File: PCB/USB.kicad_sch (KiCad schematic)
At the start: 7 parts, among them U20 xc7z020clg484

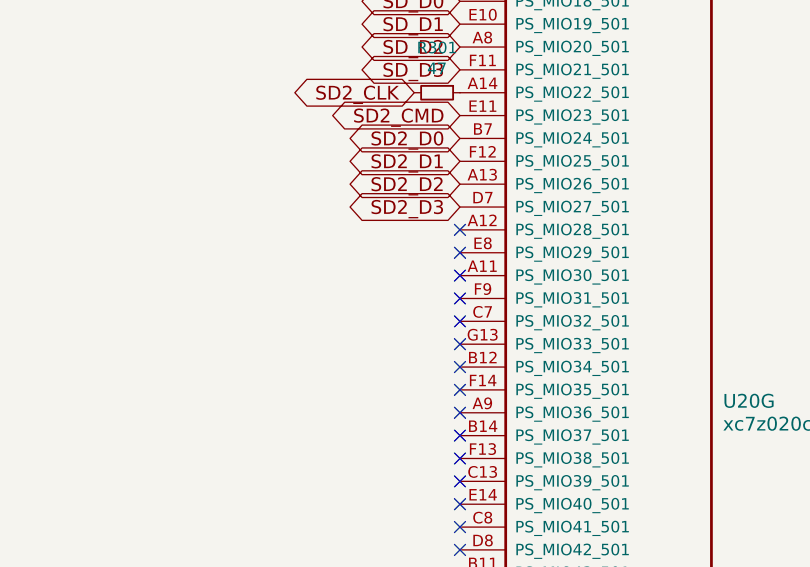
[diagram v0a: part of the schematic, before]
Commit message: some changes
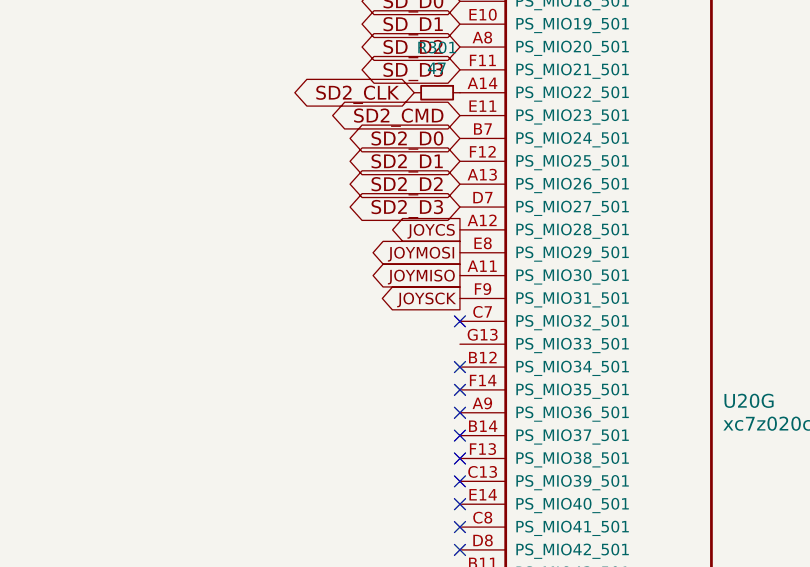
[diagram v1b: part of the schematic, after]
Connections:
- net JOYMISO: now reaches U20.A11 (PS_MIO30_501)
- net JOYCS: now reaches U20.A12 (PS_MIO28_501)
- net JOYMOSI: now reaches U20.E8 (PS_MIO29_501)
- net JOYSCK: now reaches U20.F9 (PS_MIO31_501)
- no-connect marks 27 -> 22
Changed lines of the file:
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@@
 	)
 	(no_connect
-		(at 125.095 92.71)
+		(at 125.095 128.27)
+	)
+	(no_connect
+		(at 125.095 140.97)
+	)
+	(no_connect
+		(at 125.095 133.35)
+	)
+	(no_connect
+		(at 125.095 156.21)
+	)
+	(no_connect
+		(at 125.095 125.73)
+	)
+	(no_connect
+		(at 125.095 148.59)
+	)
+	(no_connect
+		(at 125.095 123.19)
+	)
+	(no_connect
+		(at 125.095 130.81)
+	)
+	(no_connect
+		(at 125.095 115.57)
+	)
+	(no_connect
+		(at 125.095 146.05)
+	)
+	(no_connect
+		(at 125.095 120.65)
+	)
+	(no_connect
+		(at 125.095 135.89)
+	)
+	(no_connect
+		(at 125.095 143.51)
 	)
 	(no_connect
@@
 	)
 	(no_connect
-		(at 125.095 128.27)
-	)
-	(no_connect
-		(at 125.095 140.97)
-	)
-	(no_connect
-		(at 125.095 133.35)
-	)
-	(no_connect
-		(at 125.095 156.21)
-	)
-	(no_connect
-		(at 125.095 125.73)
-	)
-	(no_connect
-		(at 125.095 148.59)
-	)
-	(no_connect
-		(at 125.095 123.19)
-	)
-	(no_connect
-		(at 125.095 130.81)
-	)
-	(no_connect
-		(at 125.095 115.57)
-	)
-	(no_connect
-		(at 125.095 146.05)
-	)
-	(no_connect
-		(at 125.095 120.65)
-	)
-	(no_connect
-		(at 125.095 97.79)
-	)
-	(no_connect
-		(at 125.095 135.89)
-	)
-	(no_connect
-		(at 125.095 100.33)
-	)
-	(no_connect
-		(at 125.095 143.51)
-	)
-	(no_connect
 		(at 125.095 153.67)
 	)
 	(no_connect
 		(at 125.095 138.43)
-	)
-	(no_connect
-		(at 125.095 105.41)
-	)
-	(no_connect
-		(at 125.095 95.25)
 	)
 	(no_connect
@@
 		)
 	)
+	(global_label "JOYCS"
+		(shape output)
+		(at 125.095 92.71 180)
+		(fields_autoplaced yes)
+		(effects
+			(font
+				(size 1.27 1.27)
+			)
+			(justify right)
+		)
+		(property "Intersheetrefs" "${INTERSHEET_REFS}"
+			(at 116.8978 92.71 0)
+			(effects
+				(font
+					(size 1.27 1.27)
+				)
+				(justify right)
+				(hide yes)
+			)
+		)
+	)
 	(global_label "SD2_D3"
 		(shape bidirectional)
@@
 		)
 	)
+	(global_label "JOYSCK"
+		(shape output)
+		(at 125.095 100.33 180)
+		(fields_autoplaced yes)
+		(effects
+			(font
+				(size 1.27 1.27)
+			)
+			(justify right)
+		)
+		(property "Intersheetrefs" "${INTERSHEET_REFS}"
+			(at 115.6278 100.33 0)
+			(effects
+				(font
+					(size 1.27 1.27)
+				)
+				(justify right)
+				(hide yes)
+			)
+		)
+	)
 	(global_label "SD2_D2"
 		(shape bidirectional)
@@
 		)
 	)
+	(global_label "JOYMISO"
+		(shape output)
+		(at 125.095 97.79 180)
+		(fields_autoplaced yes)
+		(effects
+			(font
+				(size 1.27 1.27)
+			)
+			(justify right)
+		)
+		(property "Intersheetrefs" "${INTERSHEET_REFS}"
+			(at 114.7811 97.79 0)
+			(effects
+				(font
+					(size 1.27 1.27)
+				)
+				(justify right)
+				(hide yes)
+			)
+		)
+	)
 	(global_label "SD2_D1"
 		(shape bidirectional)
@@
 				(hide yes)
 			)
+		)
+	)
+	(global_label "JOYMOSI"
+		(shape output)
+		(at 125.095 95.25 180)
+		(fields_autoplaced yes)
+		(effects
+			(font
+				(size 1.27 1.27)
+			)
+			(justify right)
+		)
+		(property "Intersheetrefs" "${INTERSHEET_REFS}"
+			(at 114.7811 95.25 0)
+			(effects
+				(font
+					(size 1.27 1.27)
+				)
+				(justify right)
+				(hide yes)
+			)

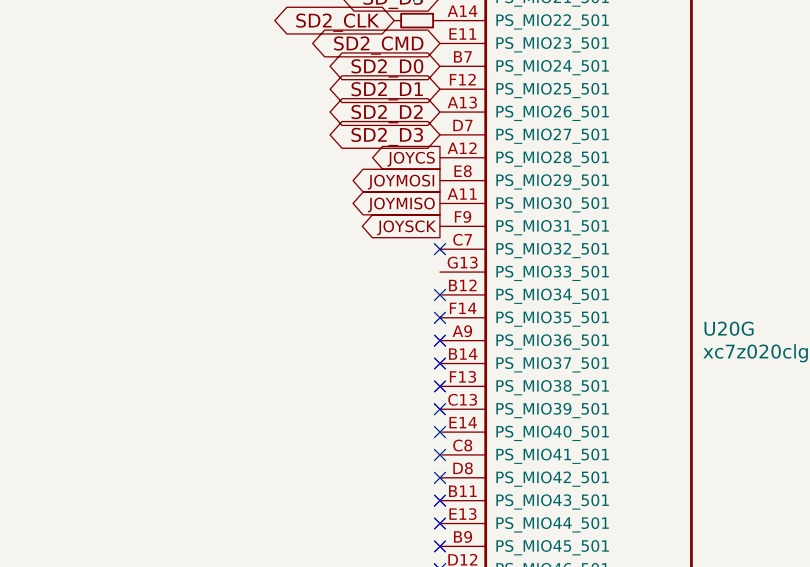
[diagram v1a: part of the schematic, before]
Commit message: [+] Layouting
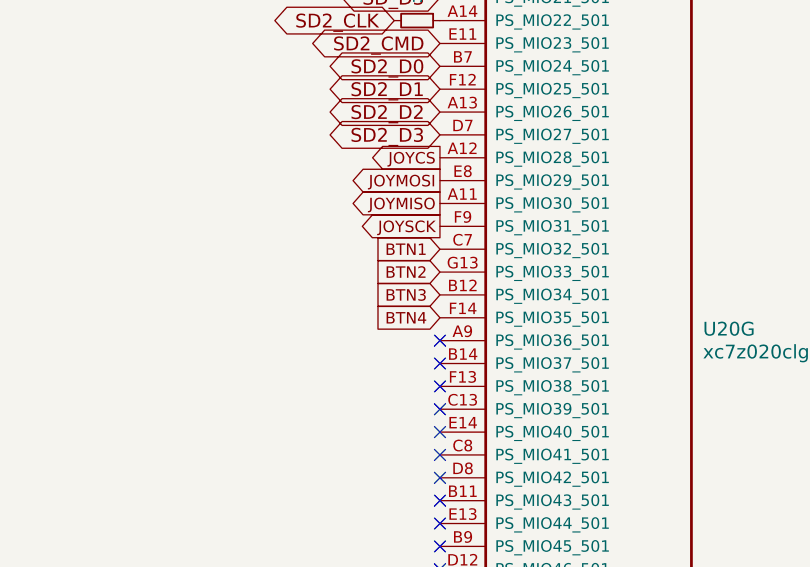
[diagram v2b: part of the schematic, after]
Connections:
- net BTN3: now reaches U20.B12 (PS_MIO34_501)
- net BTN1: now reaches U20.C7 (PS_MIO32_501)
- net BTN4: now reaches U20.F14 (PS_MIO35_501)
- net BTN2: now reaches U20.G13 (PS_MIO33_501)
- no-connect marks 22 -> 19
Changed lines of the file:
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@@
-	)
-	(no_connect
-		(at 125.095 107.95)
 	)
 	(no_connect
@@
 	)
 	(no_connect
-		(at 125.095 102.87)
-	)
-	(no_connect
 		(at 125.095 153.67)
 	)
 	(no_connect
 		(at 125.095 138.43)
-	)
-	(no_connect
-		(at 125.095 110.49)
 	)
 	(wire
@@
 		)
 	)
+	(global_label "BTN4"
+		(shape input)
+		(at 125.095 110.49 180)
+		(fields_autoplaced yes)
+		(effects
+			(font
+				(size 1.27 1.27)
+			)
+			(justify right)
+		)
+		(property "Intersheetrefs" "${INTERSHEET_REFS}"
+			(at 117.9864 110.49 0)
+			(effects
+				(font
+					(size 1.27 1.27)
+				)
+				(justify right)
+				(hide yes)
+			)
+		)
+	)
 	(global_label "SD_D1"
 		(shape bidirectional)
@@
 		)
 	)
+	(global_label "BTN1"
+		(shape input)
+		(at 125.095 102.87 180)
+		(fields_autoplaced yes)
+		(effects
+			(font
+				(size 1.27 1.27)
+			)
+			(justify right)
+		)
+		(property "Intersheetrefs" "${INTERSHEET_REFS}"
+			(at 117.9864 102.87 0)
+			(effects
+				(font
+					(size 1.27 1.27)
+				)
+				(justify right)
+				(hide yes)
+			)
+		)
+	)
 	(global_label "SD_CMD"
 		(shape bidirectional)
@@
 					(size 1.27 1.27)
 				)
+				(hide yes)
+			)
+		)
+	)
+	(global_label "BTN2"
+		(shape input)
+		(at 125.095 105.41 180)
+		(fields_autoplaced yes)
+		(effects
+			(font
+				(size 1.27 1.27)
+			)
+			(justify right)
+		)
+		(property "Intersheetrefs" "${INTERSHEET_REFS}"
+			(at 117.9864 105.41 0)
+			(effects
+				(font
+					(size 1.27 1.27)
+				)
+				(justify right)
 				(hide yes)
 			)
@@
 			(effects
 				(font
+					(size 1.27 1.27)
+				)
+				(justify right)
+				(hide yes)
+			)
+		)
+	)
+	(global_label "BTN3"
+		(shape input)
+		(at 125.095 107.95 180)
+		(fields_autoplaced yes)
+		(effects
+			(font
+				(size 1.27 1.27)
+			)
+			(justify right)
+		)
+		(property "Intersheetrefs" "${INTERSHEET_REFS}"
+			(at 117.9864 107.95 0)
+			(effects
+				(font
